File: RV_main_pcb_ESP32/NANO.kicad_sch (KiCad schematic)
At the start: 18 parts, among them J10 USB_B_Micro, SW1 SW_Push, U6 ATmega328P-A, U7 FT232RL, Y2 Crystal_GND2

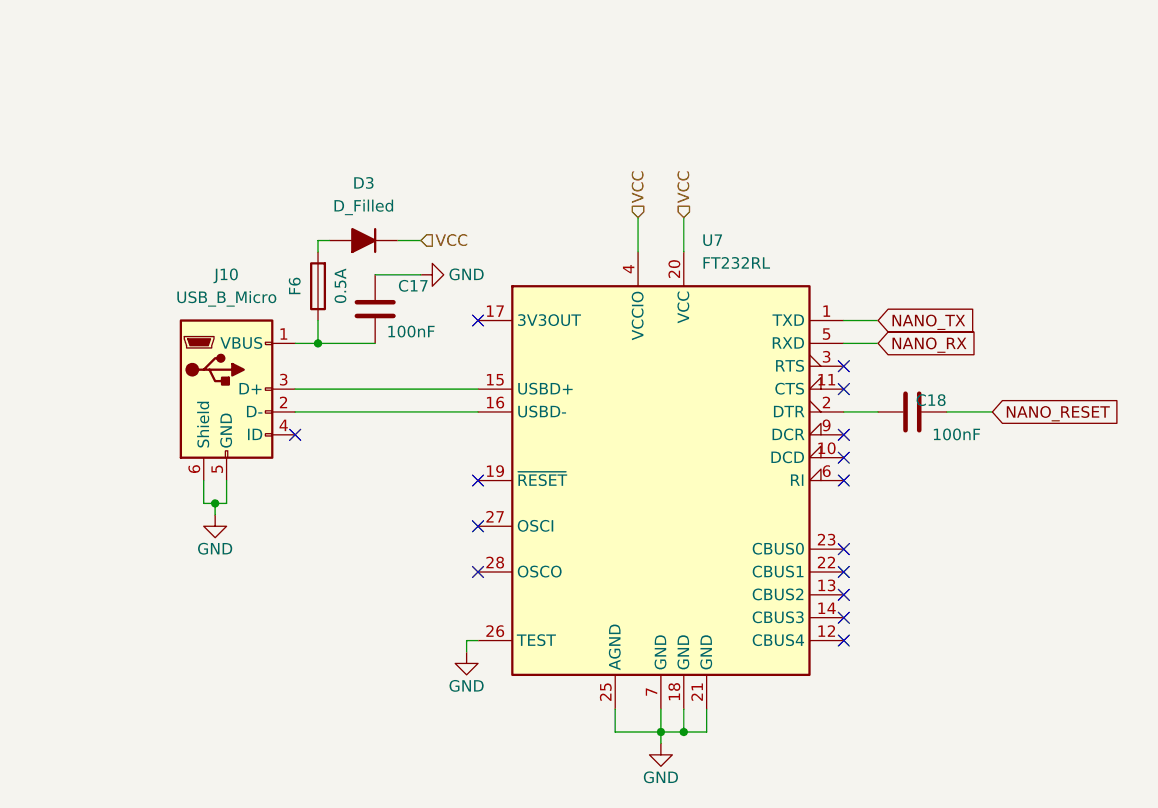
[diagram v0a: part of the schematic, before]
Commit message: update
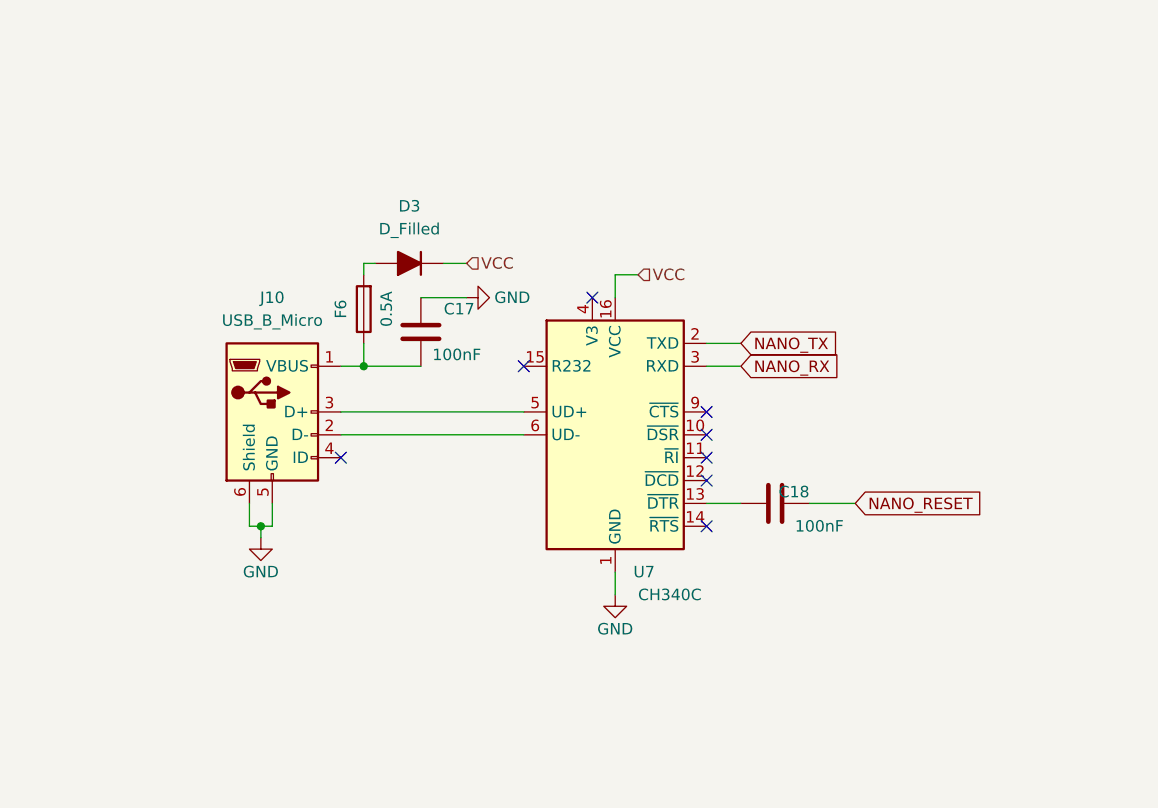
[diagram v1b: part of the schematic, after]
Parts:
- removed U7: FT232RL, Package_SO:SSOP-28_5.3x10.2mm_P0.65mm, symbol Interface_USB:FT232RL
- added U7: CH340C, Package_SO:SOIC-16_3.9x9.9mm_P1.27mm, symbol Interface_USB:CH340C
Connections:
- net GND: now also U7.1 (GND)
- net NANO_RX: now also U7.3 (RXD)
- net NANO_TX: now also U7.2 (TXD)
- net VCC: now also U7.16 (VCC)
- net at C18.1: now also U7.13 (~{DTR})
- net at J10.3 (D+): now also U7.5 (UD+)
- net at J10.2 (D-): now also U7.6 (UD-)
- no-connect marks 21 -> 14
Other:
- moved on the sheet: C17, C18, D3, F6, J10
